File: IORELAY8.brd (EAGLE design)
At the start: 64.8 x 46.7 mm, 55 parts, among them Q1 2N7002, Q2 2N7002, Q3 2N7002, Q4 2N7002, Q5 2N7002, Q6 2N7002, Q7 2N7002, Q8 2N7002

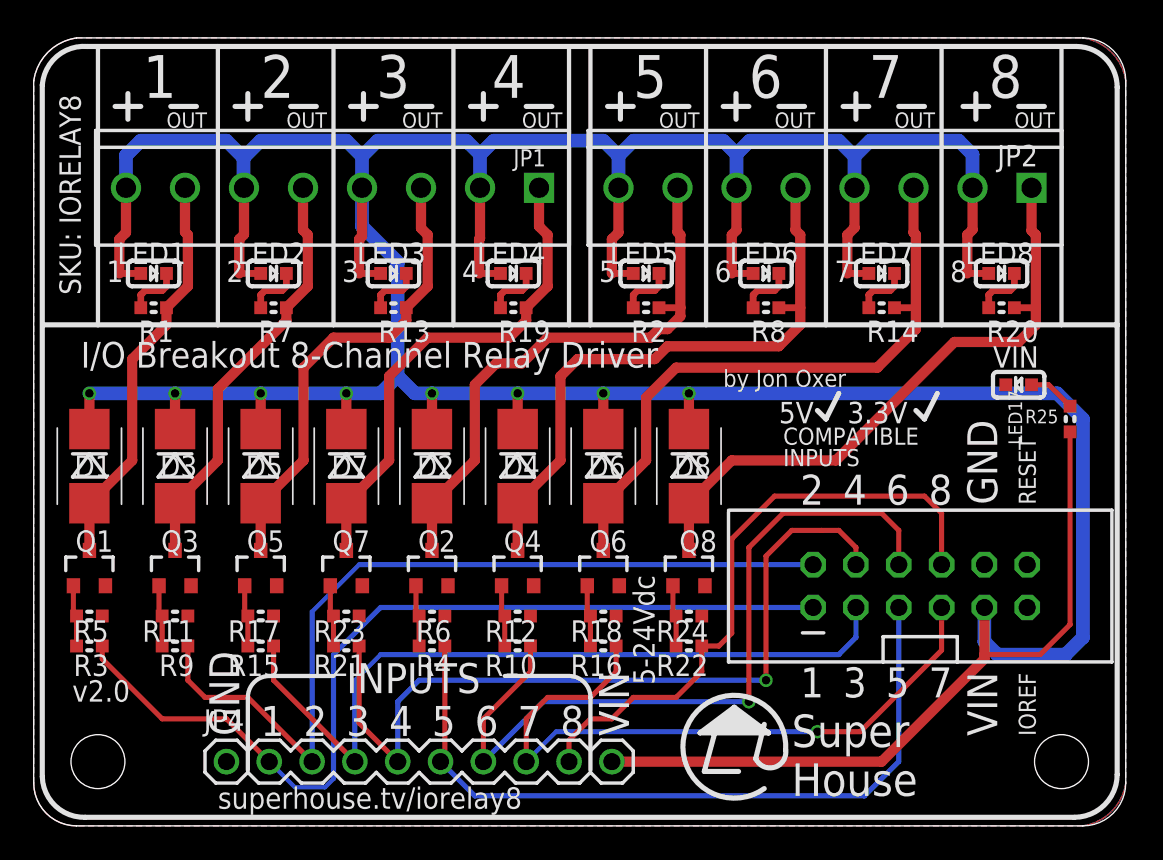
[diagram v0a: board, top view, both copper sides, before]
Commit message: Resized board on metric grid
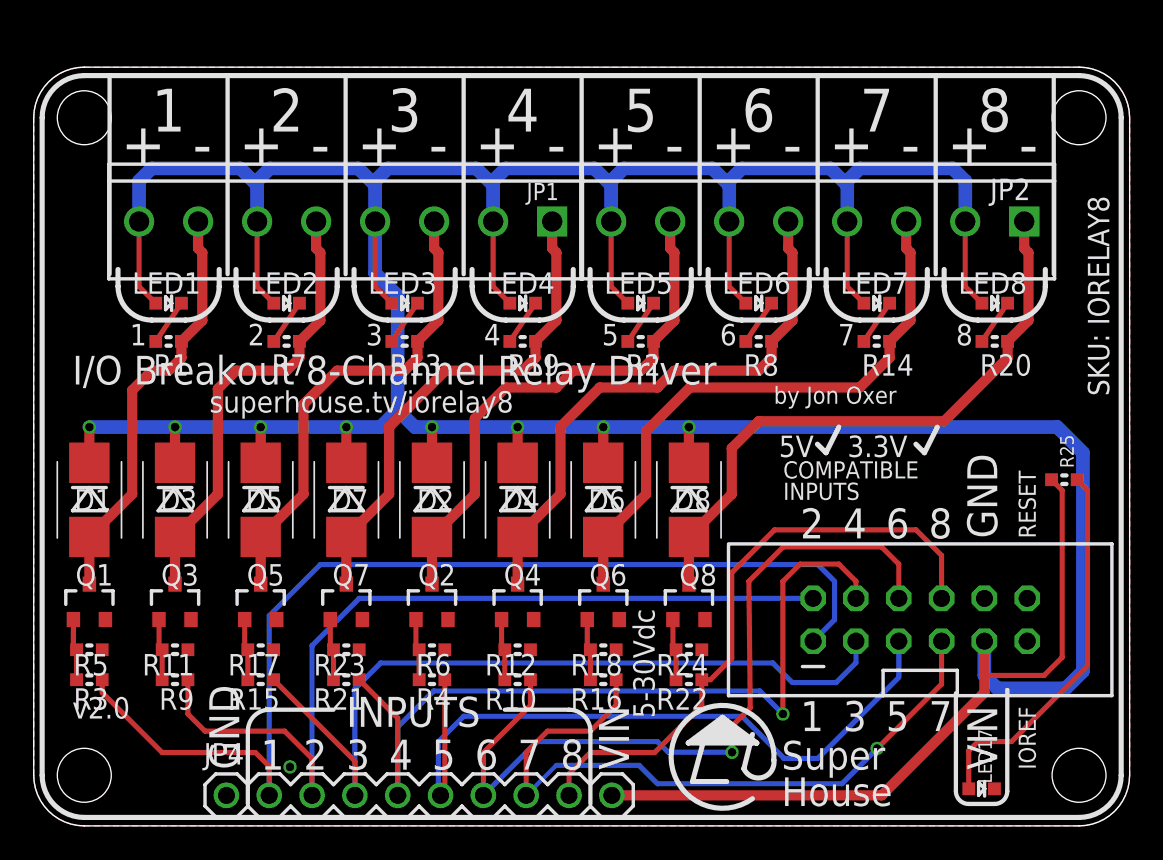
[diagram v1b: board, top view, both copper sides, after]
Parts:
- moved LED17 24.1 mm to (56.2, 2.20), turned to 0 degrees
- moved R25 3.61 mm to (61.1, 20.5), turned to 180 degrees
- moved R1 2.19 mm to (8.00, 28.7)
- moved JP1 2.15 mm to (30.8, 35.8)
- moved R7 2.15 mm to (15.0, 28.7)
- moved R13 2.11 mm to (22.0, 28.7)
- moved R19 2.07 mm to (29.0, 28.7)
- moved R8 2.05 mm to (43.0, 28.7)
- moved JP2 2.05 mm to (58.8, 35.8)
- moved R20 2.04 mm to (57.0, 28.7)
- moved R2 2.03 mm to (36.0, 28.7)
- moved R14 2.02 mm to (50.0, 28.7)
- moved D1 2.00 mm to (3.30, 19.3)
- moved D2 2.00 mm to (23.6, 19.3)
- moved D3 2.00 mm to (8.38, 19.3)
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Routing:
- net N$4: track 2.81 -> 22.7 mm
- net D0: track 54.8 -> 64.1 mm
- net VCC: track 278.3 -> 269.4 mm
- net N$15: track 36.4 -> 33.3 mm
- net N$17: track 37.6 -> 35.1 mm
- net N$3: track 25.1 -> 27.1 mm
- net N$13: track 33.7 -> 31.7 mm
- net D3: track 48.5 -> 50.2 mm
- net D4: track 45.0 -> 43.3 mm
- net D2: track 46.2 -> 47.8 mm
- net D1: track 51.2 -> 52.4 mm
- net N$5: track 24.0 -> 25.0 mm
- net D6: track 40.5 -> 41.4 mm
- net N$19: track 37.3 -> 36.5 mm
- net N$9: track 27.9 -> 28.5 mm
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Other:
- board size 64.8 x 46.7 mm -> 65 x 45 mm
- board text added: "+"
- board text added: "-"
- board text added: "5-30Vdc"
- board text removed: "5-24Vdc"
- board text removed: "OUT"
